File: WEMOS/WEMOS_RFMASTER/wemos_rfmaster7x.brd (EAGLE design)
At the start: 45.7 x 37.5 mm, 14 parts

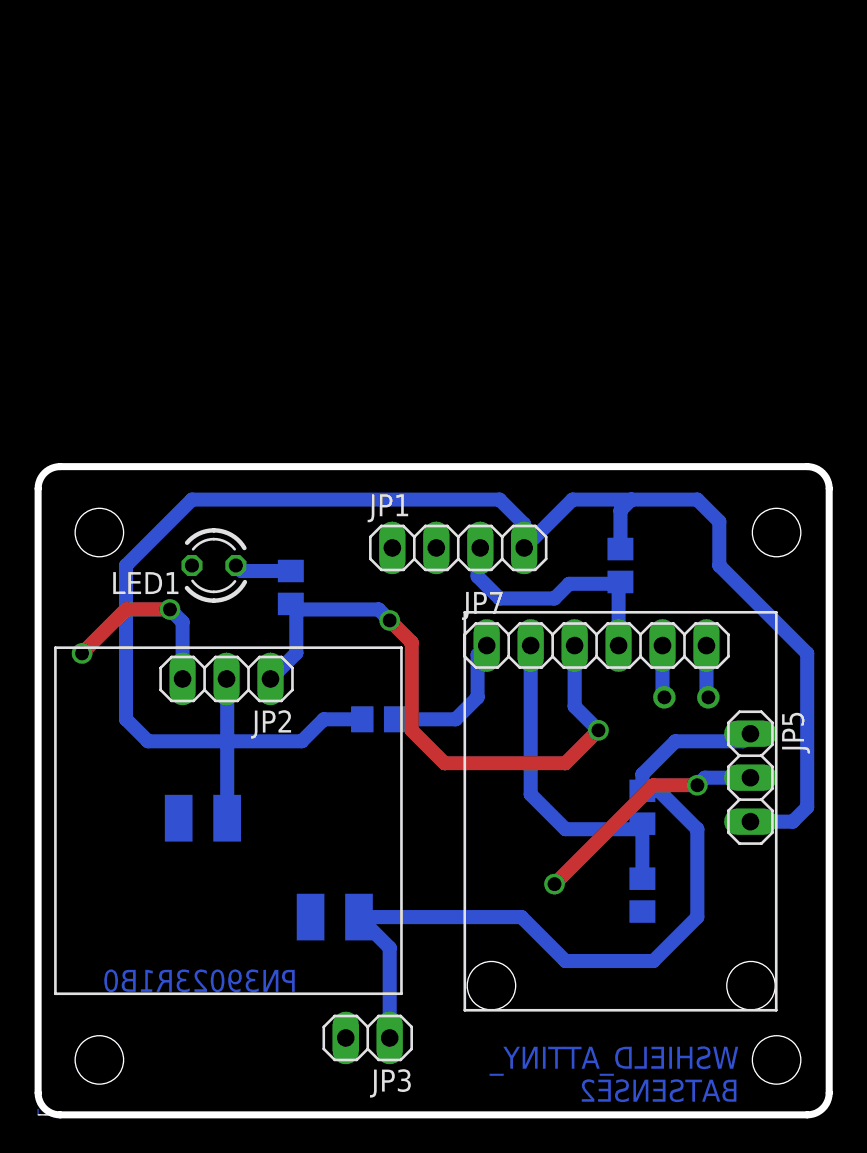
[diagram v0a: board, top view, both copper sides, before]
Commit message: updated boards and wirings
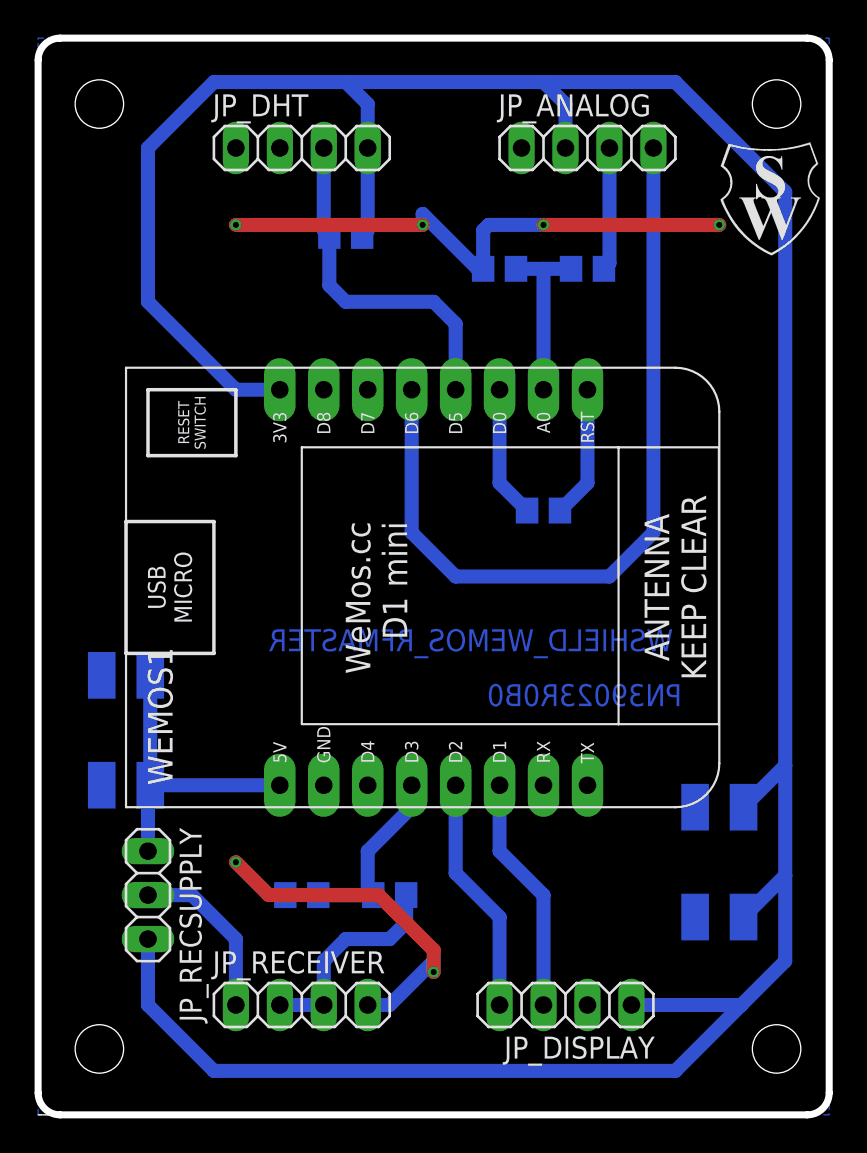
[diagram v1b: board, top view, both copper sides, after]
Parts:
- removed JP1: (no value), pinhead:1X04
- removed JP2, JP5: (no value), pinhead:1X03
- removed JP3: (no value), pinhead:1X02
- removed JP7: (no value), pinhead:1X06
- removed LED1: (no value), led:LED3MM
- added C2, C4: (no value), rcl:C1210
- added JP_ANALOG, JP_DISPLAY, JP_RECEIVER: (no value), pinhead:1X04
- added JP_DHT: (no value), pinhead@1:1X04
- added JP_RECSUPPLY: (no value), pinhead@1:1X03
- added R6: 10k, rcl:R0805
- added WEMOS1: (no value), SWI_COMMONS:WEMOS-D1-MINI
- R1: value 10k -> 470Ohm
- R2, R3, R4, R5: value 10k -> (none)
- moved U$2 40.4 mm to (39.2, 49.5), flipped to the top
- moved R5 37.1 mm to (26.7, 48.9), turned to 180 degrees
- moved R4 31.3 mm to (31.8, 48.9), turned to 180 degrees
- moved R2 23.3 mm to (20.3, 12.7), turned to 180 degrees
- moved C3 23.1 mm to (39.4, 17.8)
- moved R3 17.8 mm to (15.2, 12.7), turned to 180 degrees
- moved R1 15.4 mm to (29.2, 34.9)
- moved C1 9.38 mm to (5.08, 25.4)
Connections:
- removed net DGND: C1.2, C3.2, JP1.1, JP2.3, JP3.2, JP5.2, LED1.K, R5.2
- removed net N$2: LED1.A, R3.2
- removed net P0: JP7.6
- removed net P1: JP7.5
- removed net P2: JP1.3, JP7.4, R2.2
- removed net P3: JP2.1, JP7.3, R3.1
- removed net P4: JP7.2, R4.2, R5.1
- removed net P5: JP7.1, R1.1
- removed net VIN: C3.1, JP3.1, JP5.1, R4.1
- new net +3V3: C3.1, C4.1, JP_ANALOG.2, JP_DHT.4, JP_DISPLAY.1, JP_RECSUPPLY.3, R6.1, WEMOS1.3V3
- new net A0: R4.1, R5.2, WEMOS1.A0
- new net AIN: JP_ANALOG.3, R4.2
- new net D0: R1.2, WEMOS1.D0
- new net D3: R2.1, R3.2, WEMOS1.D3
- new net D4: WEMOS1.D4
- new net D5: JP_DHT.3, R6.2, WEMOS1.D5
- new net D6: JP_ANALOG.4, WEMOS1.D6
- new net D7: WEMOS1.D7
- new net D8: WEMOS1.D8
- new net GND: C1.2, C2.2, C3.2, C4.2, JP_ANALOG.1, JP_DHT.1, JP_DISPLAY.2, JP_RECEIVER.4, R3.1, R5.1, WEMOS1.GND
- new net RESET: R1.1, WEMOS1.RESET
- new net RIN: JP_RECEIVER.1, JP_RECSUPPLY.2
- new net ROUT: JP_RECEIVER.2, JP_RECEIVER.3, R2.2
- new net RX: WEMOS1.RX
- new net SCA: JP_DISPLAY.4, WEMOS1.D2
- new net SCL: JP_DISPLAY.3, WEMOS1.D1
- new net TX: WEMOS1.TX
- net +5V: now also C2.1, JP_RECSUPPLY.1, WEMOS1.5V; no longer JP1.4, JP2.2, JP5.3, R1.2, R2.1
- net NA: now also JP_DHT.2; no longer JP1.2
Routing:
- net +3V3: track 0.00 -> 176.0 mm
- net +5V: track 96.6 -> 17.7 mm
- net GND: track 0.00 -> 52.5 mm, vias 0 -> 6
- net VIN: track 46.7 -> 0.00 mm
- net D6: track 0.00 -> 46.6 mm
- net P3: track 35.5 -> 0.00 mm, vias 2 -> 0
- net DGND: track 24.3 -> 0.00 mm, vias 4 -> 0
- net D5: track 0.00 -> 20.1 mm
- net P4: track 19.2 -> 0.00 mm
- net P2: track 14.5 -> 0.00 mm
- net SCA: track 0.00 -> 13.8 mm
- net SCL: track 0.00 -> 13.8 mm
- net ROUT: track 0.00 -> 12.3 mm
- net D3: track 0.00 -> 10.7 mm
- net A0: track 0.00 -> 10.2 mm
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- added copper zone on layer 16, net GND
- removed copper zone on layer 16, net DGND
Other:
- board size 45.7 x 37.5 mm -> 45.7 x 62.2 mm
- board text added: "PN39023R0B0"
- board text added: "WSHIELD_WEMOS_RFMASTER"
- board text removed: "PN39023R1B0"
- board text removed: "WSHIELD_ATTINY_ BATSENSE2"
